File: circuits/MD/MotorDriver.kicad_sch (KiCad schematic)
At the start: 79 parts, among them Q1 TPH3R704PL, Q2 TPH3R704PL, Q3 TPH3R704PL, Q4 TPH3R704PL, Q5 TPH3R704PL, Q6 TPH3R704PL, U1 Driver_FETGate_DRV8323x

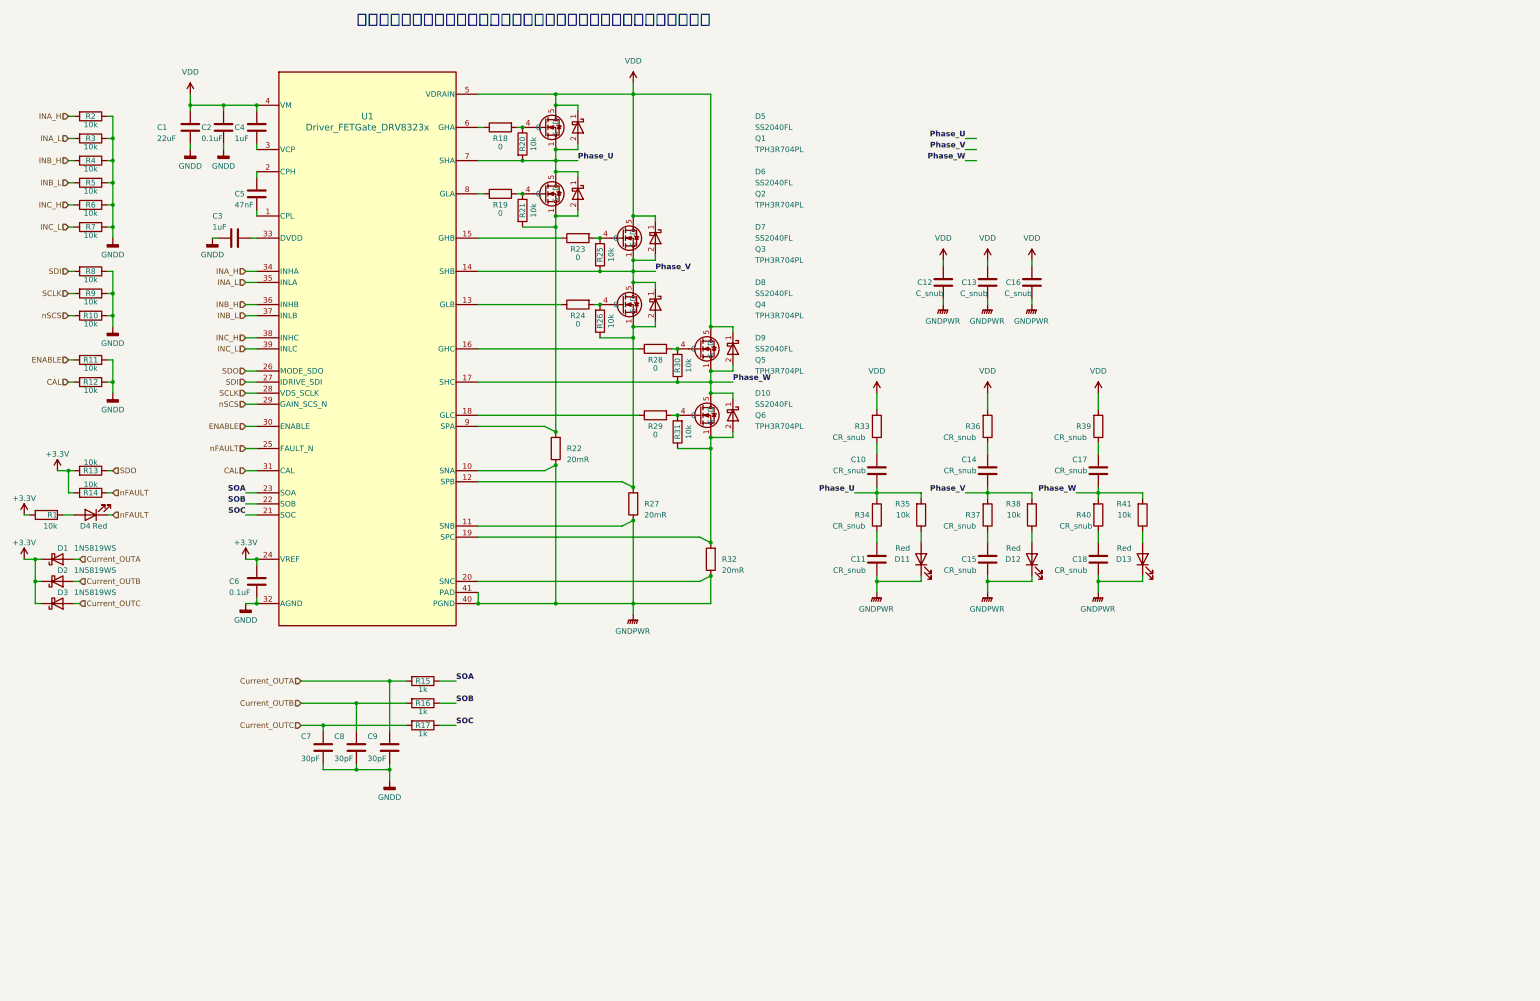
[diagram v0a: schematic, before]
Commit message: こみっと
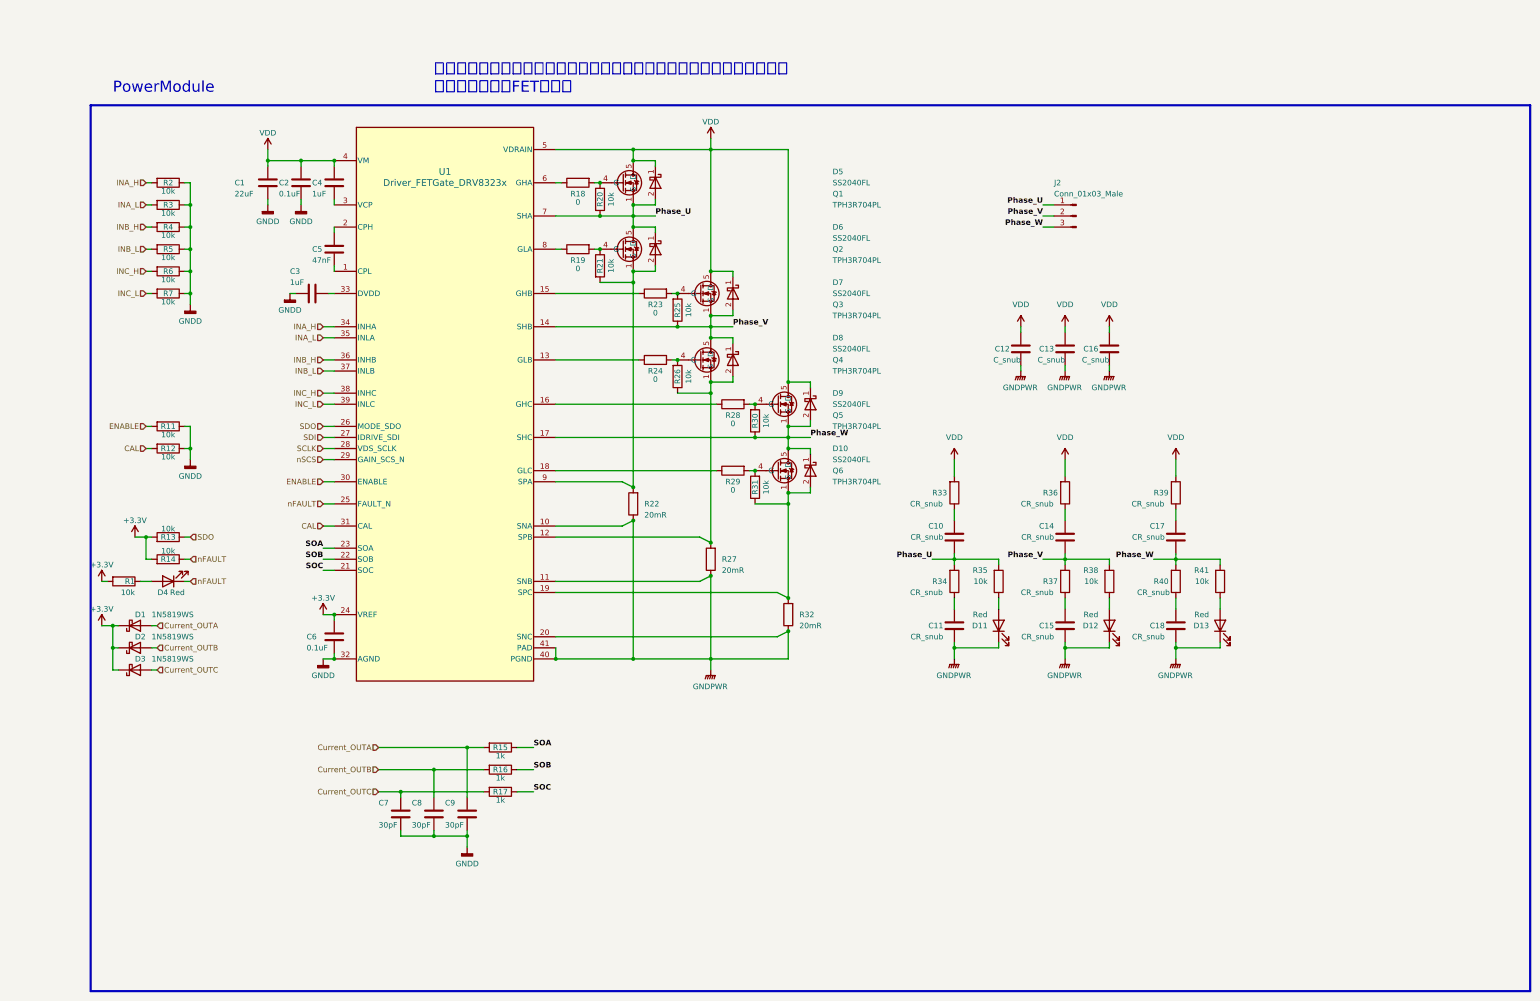
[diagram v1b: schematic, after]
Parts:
- removed R10, R8, R9: 10k, Resistor_SMD:R_0402_1005Metric, symbol Device:R
- added J2: Conn_01x03_Male, Connector_Molex:Molex_SPOX_5268-03A_1x03_P2.50mm_Horizontal, symbol Connector:Conn_01x03_Male
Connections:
- net Phase_U: now also J2.1 (Pin_1)
- net Phase_V: now also J2.2 (Pin_2)
- net Phase_W: now also J2.3 (Pin_3)
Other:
- note added: "PowerModule"
- note added: "電流センスアンプは差動電圧はどこまでいけるのか？電流最大値の設計 ハーフブリッジFETかえる"
- note removed: "電流センスアンプは差動電圧はどこまでいけるのか？電流最大値の設計"
- moved on the sheet: C1, C10, C11, C12, C13, C14, C15, C16, C17, C18, C2, C3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
